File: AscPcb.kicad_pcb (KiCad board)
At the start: 2 copper layers, 27.9 x 36.2 mm, 31 parts, among them J1 12402012E212A, J2 B2B-PH-K-S(LF)(SN), J3 Conn_01x10_Pin, SW1 TL3305AF260QG, SW2 TL3305AF260QG, U1 ESP32-C3-WROOM-02-N4, U2 BQ24040DSQR, U3 TLV75801PDRVR

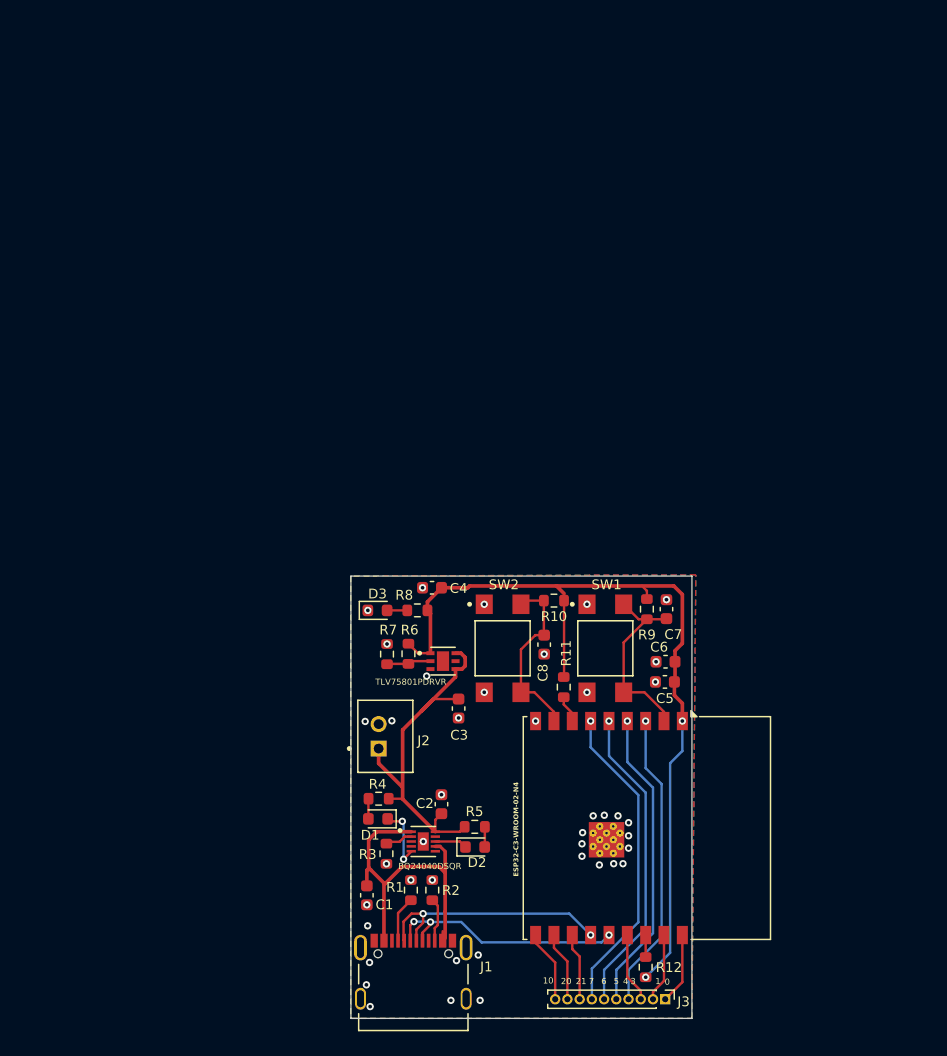
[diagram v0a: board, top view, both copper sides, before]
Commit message: motor control circuit done
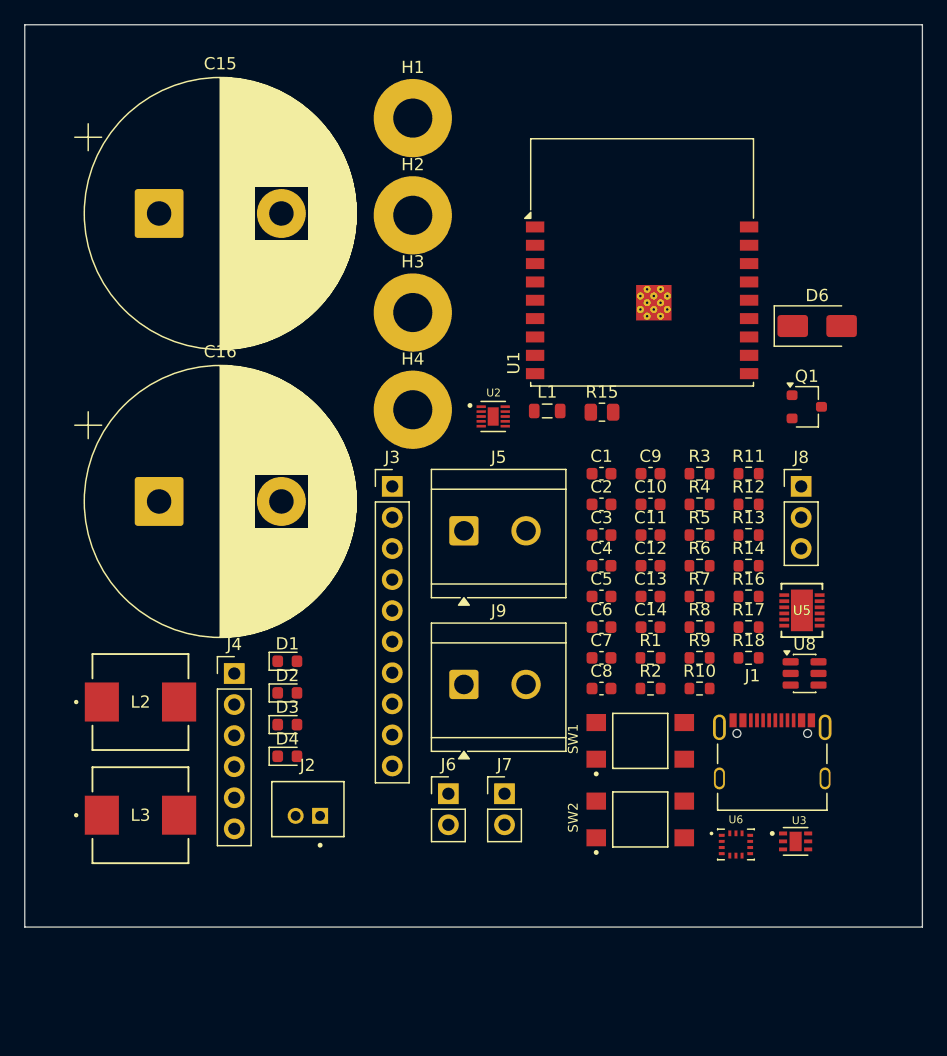
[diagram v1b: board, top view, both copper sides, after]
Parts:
- added C10: 220nF, Capacitor_SMD:C_0603_1608Metric, F.Cu at (148.5, 85.6)
- added C11: 100nF, Capacitor_SMD:C_0603_1608Metric, F.Cu at (148.5, 88.1)
- added C12: 22uF, Capacitor_SMD:C_0603_1608Metric, F.Cu at (148.5, 90.6)
- added C13: 22uF, Capacitor_SMD:C_0603_1608Metric, F.Cu at (148.5, 93.1)
- added C14: 10uF, Capacitor_SMD:C_0603_1608Metric, F.Cu at (148.5, 95.6)
- added C15: 100F, Capacitor_THT:CP_Radial_D22.0mm_P10.00mm_SnapIn, F.Cu at (108.3, 61.8)
- added C16: 100F, Capacitor_THT:CP_Radial_D22.0mm_P10.00mm_SnapIn, F.Cu at (108.3, 85.3)
- added C9: 10uF, Capacitor_SMD:C_0603_1608Metric, F.Cu at (148.5, 83.1)
- added D4: GREEN, LED_SMD:LED_0603_1608Metric, F.Cu at (118.8, 106.2)
- added D6: D_Schottky, Diode_SMD:D_SMA, F.Cu at (162.1, 71.0)
- added H1: MountingHole_Pad, MountingHole:MountingHole_3.2mm_M3_Pad, F.Cu at (129.0, 54.0)
- added H2: MountingHole_Pad, MountingHole:MountingHole_3.2mm_M3_Pad, F.Cu at (129.0, 61.9)
- added H3: MountingHole_Pad, MountingHole:MountingHole_3.2mm_M3_Pad, F.Cu at (129.0, 69.9)
- added H4: MountingHole_Pad, MountingHole:MountingHole_3.2mm_M3_Pad, F.Cu at (129.0, 77.8)
- added J4: Conn_01x06_Pin, Connector_PinHeader_2.54mm:PinHeader_1x06_P2.54mm_Vertical, F.Cu at (114.4, 99.4)
- added J5: Screw_Terminal_01x02, TerminalBlock_CUI:TerminalBlock_CUI_TB007-508-02_1x02_P5.08mm_Horizontal, F.Cu at (133.2, 87.7)
- added J6: Conn_01x02_Pin, Connector_PinHeader_2.54mm:PinHeader_1x02_P2.54mm_Vertical, F.Cu at (131.9, 109.2)
- added J7: Conn_01x02_Pin, Connector_PinHeader_2.54mm:PinHeader_1x02_P2.54mm_Vertical, F.Cu at (136.5, 109.2)
- added J8: Conn_01x03_Pin, Connector_PinHeader_2.54mm:PinHeader_1x03_P2.54mm_Vertical, F.Cu at (160.8, 84.1)
- added J9: Screw_Terminal_01x02, TerminalBlock_CUI:TerminalBlock_CUI_TB007-508-02_1x02_P5.08mm_Horizontal, F.Cu at (133.2, 100.3)
- added L1: 3.3uH, Inductor_SMD:L_0805_2012Metric, F.Cu at (140.0, 77.9)
- added L2: 3.3uH, DR73-3R3-R:DR73-3R3-R_EAT, F.Cu at (106.7, 101.7)
- added L3: 3.3uH, DR73-3R3-R:DR73-3R3-R_EAT, F.Cu at (106.7, 111.0)
- added Q1: Q_NMOS_DGS, DMN1019USN-13:SC-59-pads-swapped, F.Cu at (161.2, 77.6)
- added R13: 10k, Resistor_SMD:R_0603_1608Metric, F.Cu at (156.5, 88.1)
- added R14: 10k, Resistor_SMD:R_0603_1608Metric, F.Cu at (156.5, 90.6)
- added R15: 33.2k, Resistor_SMD:R_0805_2012Metric, F.Cu at (144.5, 78.0)
- added R16: 10k, Resistor_SMD:R_0603_1608Metric, F.Cu at (156.5, 93.1)
- added R17: 150, Resistor_SMD:R_0603_1608Metric, F.Cu at (156.5, 95.6)
- added R18: 61.9k, Resistor_SMD:R_0603_1608Metric, F.Cu at (156.5, 98.1)
- added U5: LTC3625EDE_PBF, LTC3625EDE_PBF:DFN-12_DE, F.Cu at (160.8, 94.2)
- added U6: BMI270, BMI270:XDCR_BMI270, F.Cu at (155.4, 113.4)
- added U8: AP62300TWU, Package_TO_SOT_SMD:TSOT-23-6, F.Cu at (161.1, 99.4)
- J3: footprint Connector_PinHeader_1.00mm:PinHeader_1x10_P1.00mm_Vertical -> Connector_PinHeader_2.54mm:PinHeader_1x10_P2.54mm_Vertical
- R6: value 10k -> 49.9k
- R7: value 49.9k -> 10k
- moved J3 47.5 mm to (127.3, 84.1), turned to 0 degrees
- moved U1 43.2 mm to (147.8, 68.9), turned to 0 degrees
- moved R3 40.3 mm to (152.5, 83.1), turned to 0 degrees
- moved C1 39.5 mm to (144.4, 83.1), turned to 0 degrees
- moved R12 38.8 mm to (156.5, 85.6), turned to 0 degrees
- moved R4 35.6 mm to (152.5, 85.6), turned to 0 degrees
- moved U2 35.2 mm to (135.6, 78.4)
- moved J1 34.4 mm to (158.4, 108.0)
- moved U3 32.4 mm to (160.3, 113.1)
- moved R5 30.1 mm to (152.5, 88.1)
- moved C2 27.8 mm to (144.4, 85.6), turned to 0 degrees
- moved R1 27.3 mm to (148.5, 98.1), turned to 0 degrees
- moved R7 26.0 mm to (152.5, 93.1), turned to 0 degrees
- moved R6 24.9 mm to (152.5, 90.6), turned to 0 degrees
- moved R2 24.3 mm to (148.5, 100.6), turned to 0 degrees
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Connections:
- C2 pad 1: POWER -> Net-(J6-Pin_2)
- J2 pad 1: POWER -> Net-(J6-Pin_2)
- R4 pad 1: POWER -> Net-(J6-Pin_2)
- R5 pad 1: POWER -> Net-(J6-Pin_2)
- U2 pad 10: POWER -> Net-(J6-Pin_2)
- U2 pad 3: unconnected-(U2-VSS-Pad3) -> GND
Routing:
- net +3V3: track 70.1 -> 0.00 mm, vias 2 -> 0
- net POWER: track 32.5 -> 0.00 mm
- net +5V: track 29.0 -> 0.00 mm
- net IO7: track 25.9 -> 0.00 mm, vias 1 -> 0
- net IO6: track 25.4 -> 0.00 mm, vias 1 -> 0
- net IO5: track 24.9 -> 0.00 mm, vias 1 -> 0
- net IO4: track 24.4 -> 0.00 mm, vias 1 -> 0
- net D+: track 20.4 -> 0.00 mm, vias 3 -> 0
- net D-: track 20.3 -> 0.00 mm, vias 2 -> 0
- net Net-(U1-EN): track 15.5 -> 0.00 mm
- net Net-(U1-IO9): track 14.8 -> 0.00 mm
- net IO10: track 5.91 -> 0.00 mm
- net IO0: track 5.83 -> 0.00 mm
- net IO20: track 5.71 -> 0.00 mm
- net IO3: track 5.71 -> 0.00 mm
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- removed copper zone on B.Cu, net GND
- removed copper zone on F.Cu, net GND
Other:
- board size 27.9 x 36.2 mm -> 73.4 x 73.8 mm
- board text removed: "0"
- board text removed: "1"
- board text removed: "10"
- board text removed: "20"
- board text removed: "21"
- board text removed: "3"
- board text removed: "4"
- board text removed: "5"
- board text removed: "6"
- board text removed: "7"
